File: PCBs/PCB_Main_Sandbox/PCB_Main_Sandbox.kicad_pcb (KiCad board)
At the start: 2 copper layers, 118 parts, among them J2 XT60-M, J3 HUB75, J4 fan connector, J5 To_Speaker_L, J6 To_Speaker_R, M1 CSD17581Q3, M2 CSD17581Q3A, Q3 Fan_NMOS, SW1 SW_Push, SW2 SW_Push, SW3 SW_Push, SW4 SW_Push, U2 ESP32-WROOM-E, U3 AMS1117-3.3, U4 LM5122MH/NOPB, U5 ESP32-WROVER-E, U6 LM4752TS, U7 PCM5102A, Y1 CB3LV-3I-40M000000, Y2 CB3LV-3I-40M000000

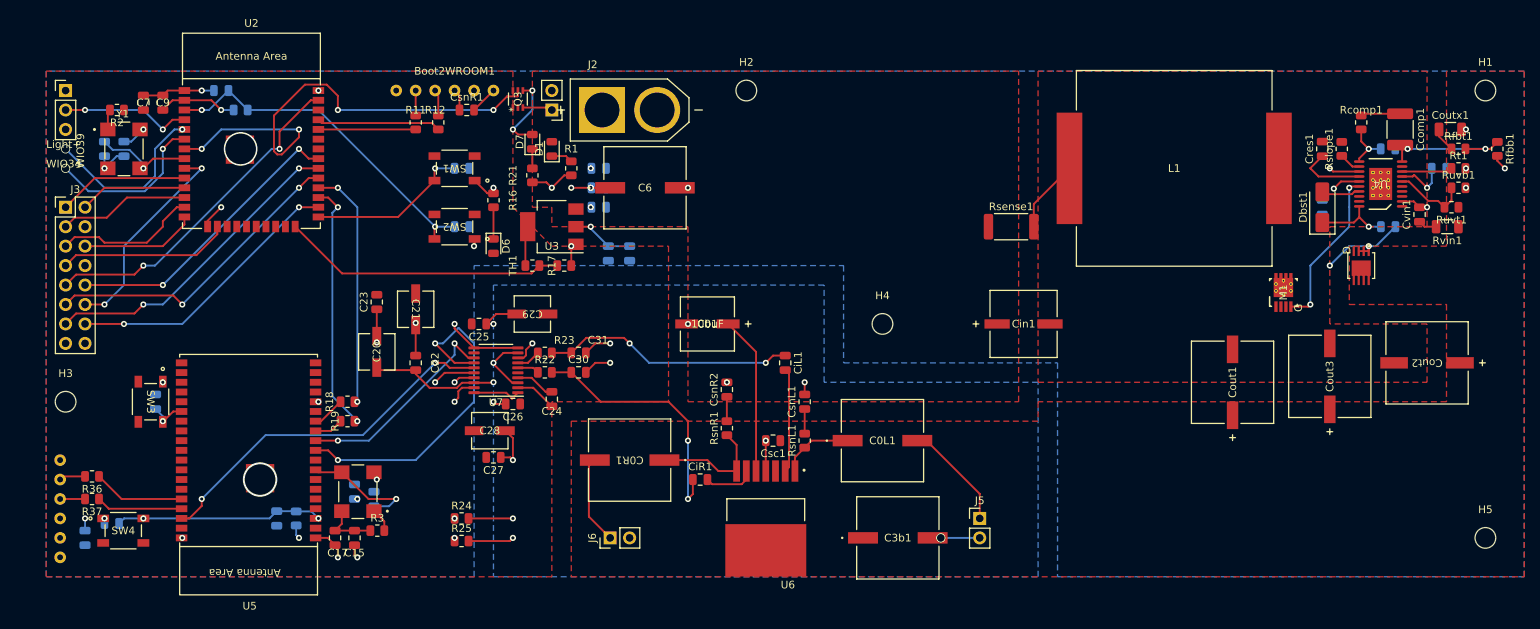
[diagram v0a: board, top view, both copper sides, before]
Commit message: Finished PCB sandbox design and added gbr and drl files
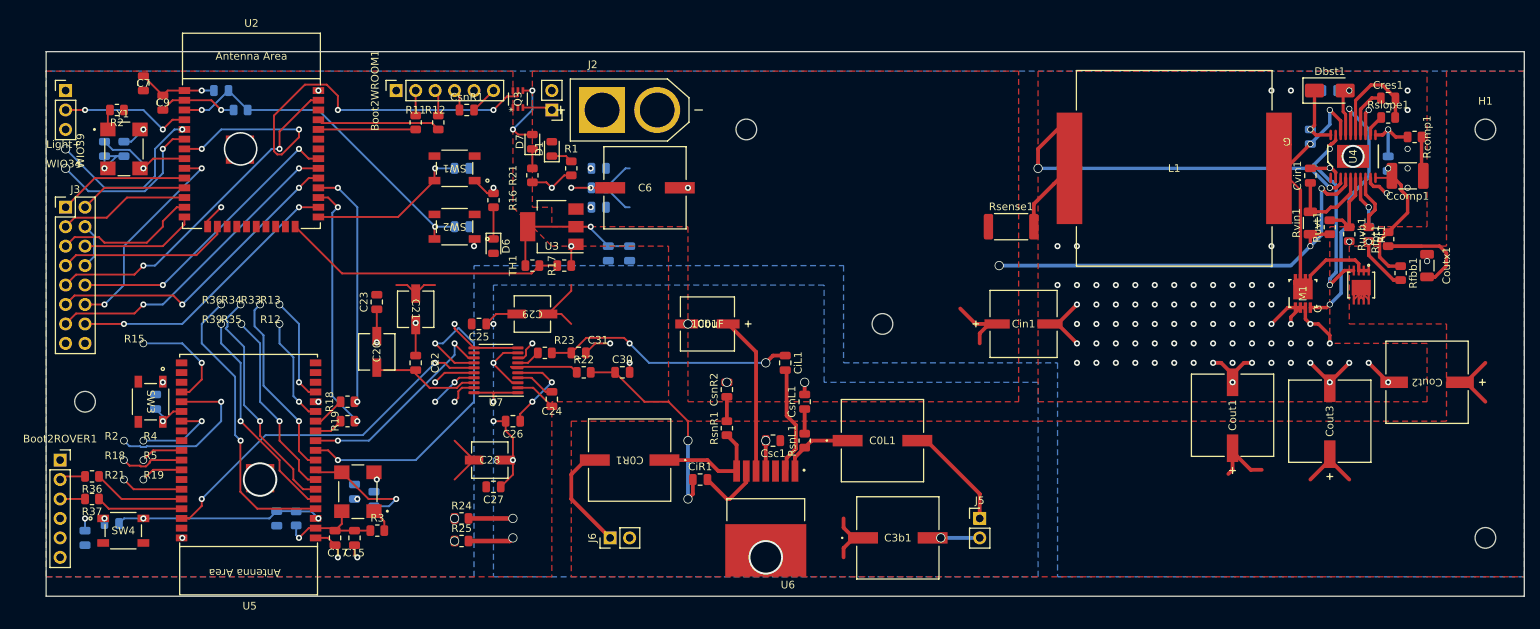
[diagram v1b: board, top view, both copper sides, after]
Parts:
- Boot2ROVER1, Boot2WROOM1: footprint Artisyn_Components:USB_TO_TTL_FT232RL -> Connector_PinSocket_2.54mm:PinSocket_1x06_P2.54mm_Vertical
- moved Rfbb1 20.6 mm to (253.1, 36.5)
- moved Coutx1 18.0 mm to (256.5, 35.6), turned to 90 degrees
- moved Rvin1 17.9 mm to (241.3, 30.0), turned to 90 degrees
- moved Ruvt1 16.1 mm to (243.8, 30.5), turned to 90 degrees
- moved Cbst1 15.5 mm to (241.3, 18.7), turned to -90 degrees
- moved Ruvb1 15.5 mm to (246.4, 31.5), turned to -90 degrees
- moved Cvcc1 15.3 mm to (243.8, 12.7), turned to 0 degrees
- moved Dbst1 15.3 mm to (243.8, 12.7), turned to 0 degrees
- moved Cvin1 15.1 mm to (241.3, 23.8)
- moved Rfbt1 14.9 mm to (251.5, 32.1), turned to 90 degrees
- moved Rt1 14.5 mm to (248.9, 31.5), turned to -90 degrees
- moved Css1 12.6 mm to (248.9, 31.4), turned to -90 degrees
- moved Cres1 10.9 mm to (251.5, 13.7), turned to 0 degrees
- moved Boot2ROVER1 7.62 mm to (78.0, 61.0)
- moved Boot2WROOM1 7.62 mm to (121.9, 12.7)
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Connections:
- Cbst1 pad 2: Net-(M1-D1) -> Net-(M1-Back)
- L1 pad 2: Net-(M1-D1) -> Net-(M1-Back)
- M1 pad 5: Net-(M1-D1) -> Net-(M1-Back)
- M1 pad 6: Net-(M1-D1) -> Net-(M1-Back)
- M1 pad 7: Net-(M1-D1) -> Net-(M1-Back)
- M1 pad 8: Net-(M1-D1) -> Net-(M1-Back)
- M1 pad 9: (no net) -> Net-(M1-Back)
- M2 pad 1: Net-(M1-D1) -> Net-(M1-Back)
- M2 pad 2: Net-(M1-D1) -> Net-(M1-Back)
- M2 pad 3: Net-(M1-D1) -> Net-(M1-Back)
- U4 pad 18: Net-(M1-D1) -> Net-(M1-Back)
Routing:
- net GND: track 81.1 -> 161.1 mm, vias 32 -> 110
- net 5V: track 5.08 -> 73.8 mm, vias 5 -> 7
- net 14V: track 3.21 -> 51.6 mm
- net Net-(U4-CSN): track 9.55 -> 57.2 mm, vias 0 -> 2
- net Net-(M1-Back): track 0.00 -> 44.3 mm, vias 0 -> 2
- net RIO36: track 0.00 -> 38.4 mm, vias 0 -> 2
- net 3.3V: track 52.9 -> 90.4 mm, vias 8 -> 10
- net RIO34: track 0.00 -> 31.0 mm, vias 0 -> 2
- net RIO39: track 0.00 -> 28.6 mm, vias 0 -> 2
- net Net-(M2-GATE): track 0.00 -> 26.5 mm, vias 0 -> 2
- net RIO35: track 0.00 -> 24.9 mm, vias 0 -> 2
- net RIO33: track 0.00 -> 24.5 mm, vias 0 -> 2
- net RIO2: track 0.00 -> 22.1 mm, vias 0 -> 2
- net RIO15: track 0.00 -> 14.2 mm, vias 0 -> 2
- net RIO13: track 0.00 -> 13.9 mm, vias 0 -> 2
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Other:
- board outline added: 193 x 71.1 mm
- board text added: "R12"
- board text added: "R13"
- board text added: "R15"
- board text added: "R18"
- board text added: "R19"
- board text added: "R2"
- board text added: "R21"
- board text added: "R33"
- board text added: "R34"
- board text added: "R35"
- board text added: "R36"
- board text added: "R39"
- board text added: "R4"
- board text added: "R5"
